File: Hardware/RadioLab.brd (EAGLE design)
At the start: 80 x 40 mm, 57 parts, among them Q1 16MHz, U1 ATMEGA32U4-AU, U2 V_REG_LDOSMD, U3 NRF24L01SMD, X3 16MHz

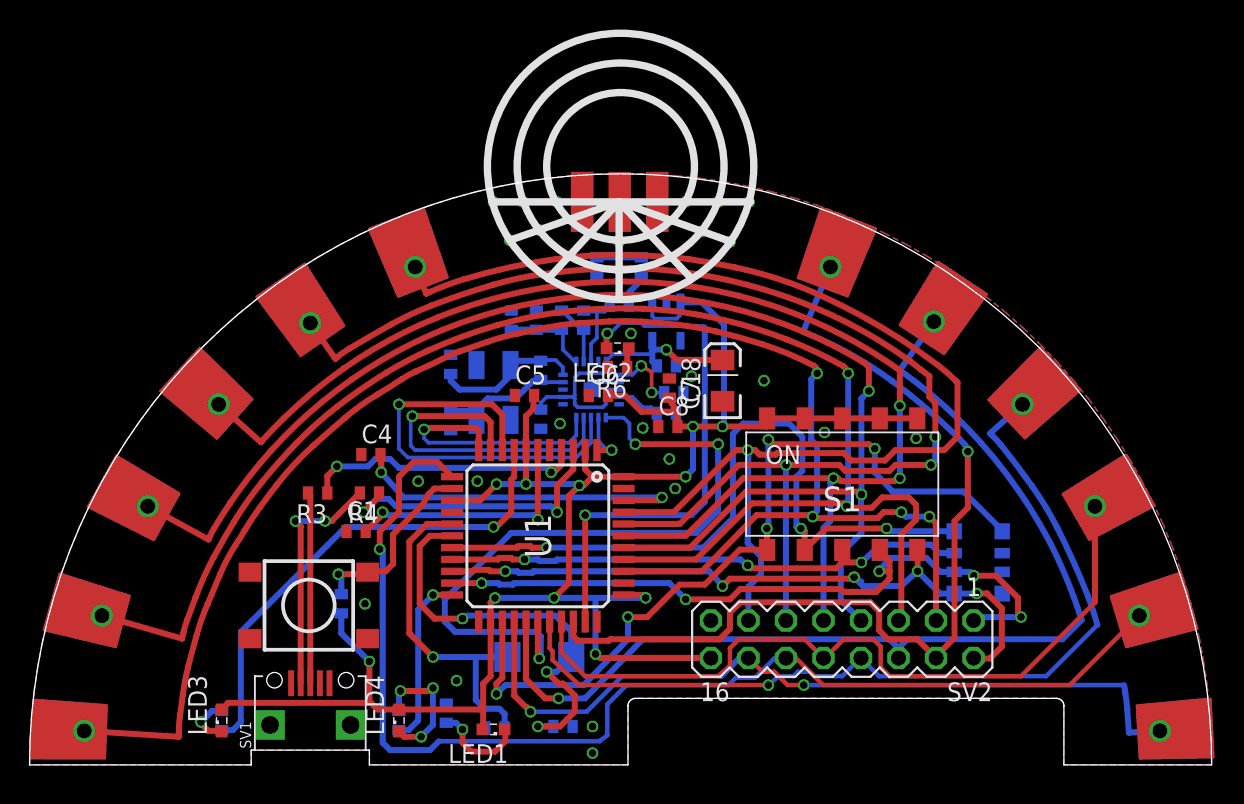
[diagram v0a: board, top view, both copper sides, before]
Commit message: Global updates
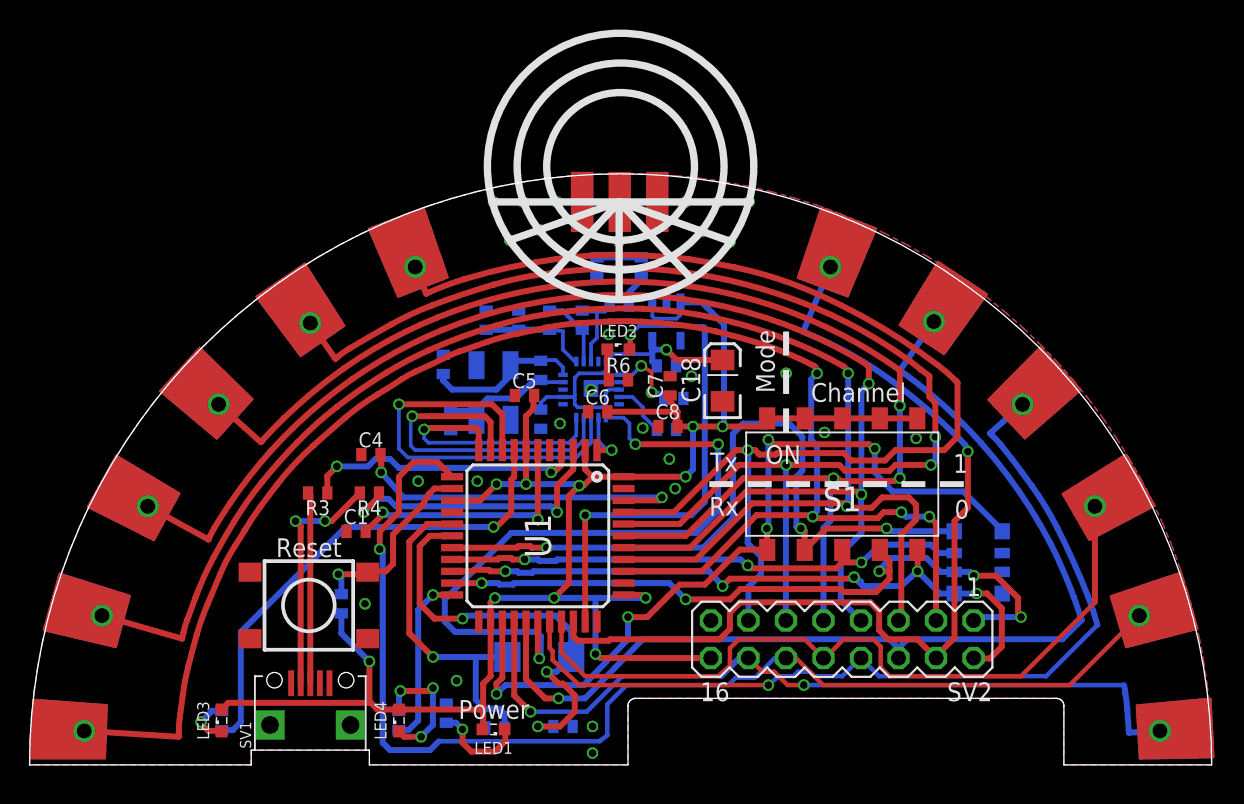
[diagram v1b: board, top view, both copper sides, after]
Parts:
- C1, C10, C11, C12, C13, C14, C15, C16, C17, C2, C3, C4, C5, C6, C7, C8, C9: device resistor:C0402 -> SpaceDIY_passive_components:0402
- L1, L2, L3: device SparkFun:C0402 -> SpaceDIY_passive_components:0402
- LED1, LED2, LED3, LED4: device led:SML0603 -> SpaceDIY_passive_components:LED0402
- R1, R2, R3, R4, R5, R6, R7, R8, R9: device resistor:R0402 -> SpaceDIY_passive_components:0402
- moved C15 1.70 mm to (30.9, 30.1)
- moved C16 1.20 mm to (33.1, 30.1)
- moved C6 1.10 mm to (38.5, 23.9)
- moved C14 1.10 mm to (43.1, 22.7)
- moved R6 0.85 mm to (39.9, 26.1), turned to 0 degrees
- moved L2 0.80 mm to (35.2, 30.1)
- moved C13 0.50 mm to (28.0, 27.1)
- moved R7 0.40 mm to (43.6, 24.8)
- moved C7 0.16 mm to (43.4, 25.6), turned to 90 degrees
- moved L3 0.10 mm to (37.4, 30.1)
- moved LED2 0.09 mm to (39.9, 28.1), turned to 0 degrees
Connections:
- net GND: now also C7.2; no longer C7.1
- net VCC: now also C7.1; no longer C7.2
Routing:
- net GND: track 2.31 -> 0.20 mm, vias 25 -> 26
- net D13: track 35.5 -> 33.8 mm
- net N$10: track 6.02 -> 7.69 mm
- net N$9: track 1.34 -> 2.18 mm
- net N$12: track 3.01 -> 3.78 mm
- net N$13: track 4.39 -> 5.09 mm
- net N$5: track 10.3 -> 10.8 mm
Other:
- board text added: "0"
- board text added: "1"
- board text added: "ANT"
- board text added: "Channel"
- board text added: "Mode"
- board text added: "Power"
- board text added: "Reset"
- board text added: "Rx"
- board text added: "Tx"
